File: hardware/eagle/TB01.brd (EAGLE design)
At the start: 50 x 50 mm, 29 parts, among them J1 CON_TERMINAL_BLOCK_02-5MM, J4 CON_TERMINAL_BLOCK_02-5MM, J5 CON_TERMINAL_BLOCK_03-5MM, T1 BT138-V, T2 BT138-V

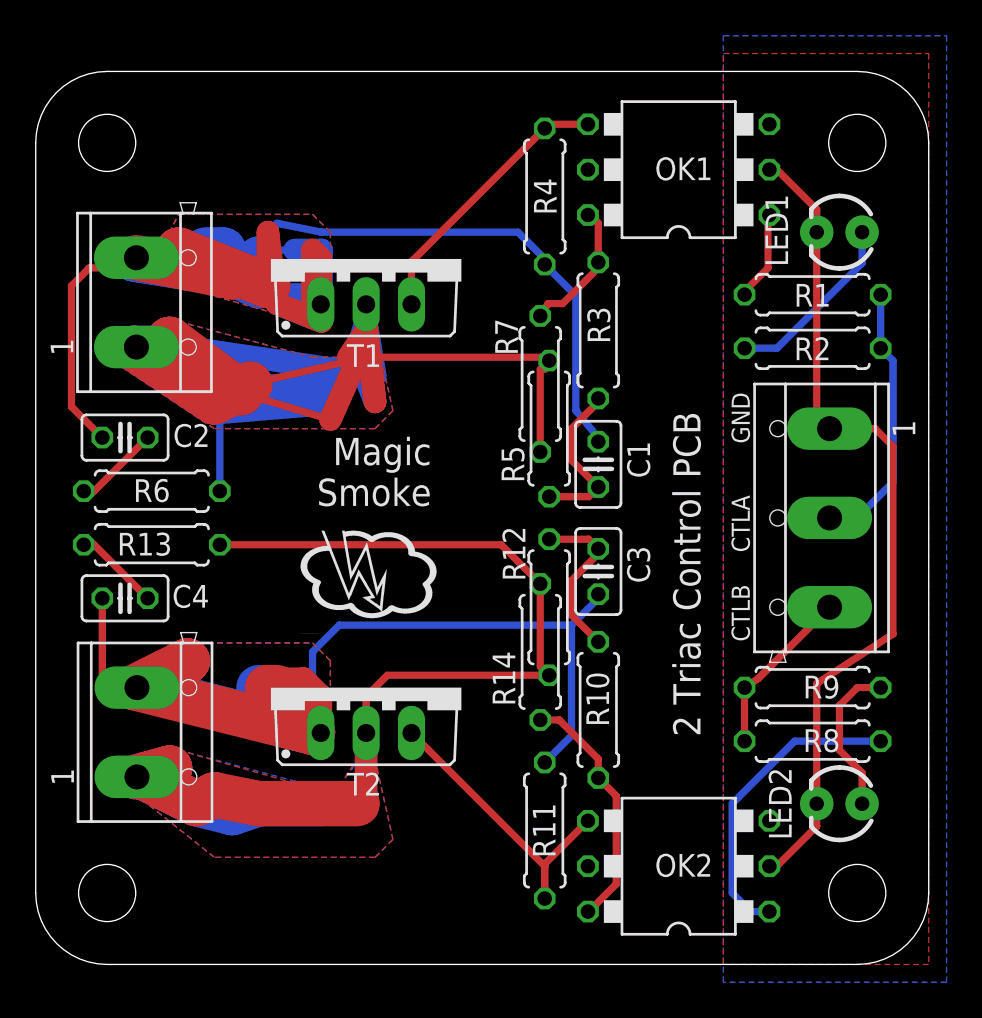
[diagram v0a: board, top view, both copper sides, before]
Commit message: high voltage warning
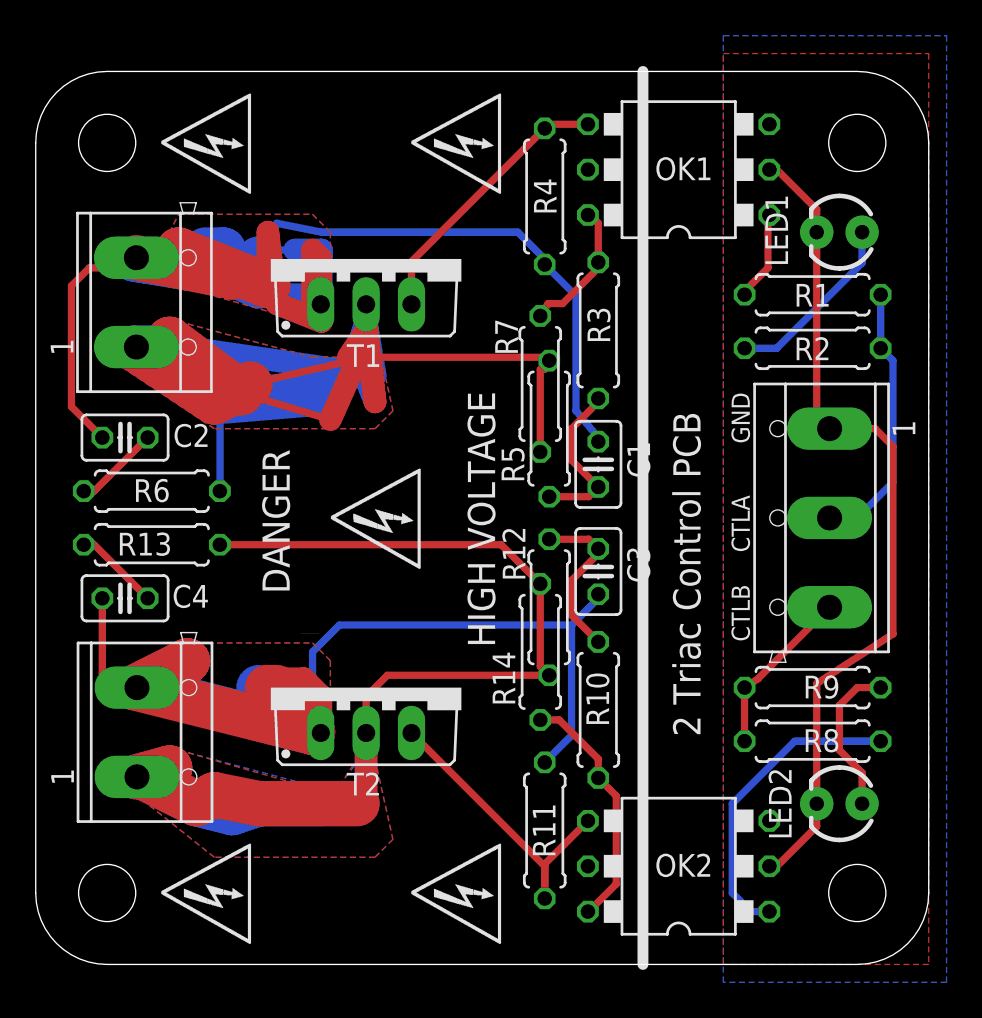
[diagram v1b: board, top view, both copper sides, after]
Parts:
- moved U$2 7.80 mm to (17.5, 25.0)
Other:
- board text added: "DANGER"
- board text added: "HIGH VOLTAGE"
- board text added: "LOAD A"
- board text added: "LOAD B"
- board text removed: "Magic Smoke"
